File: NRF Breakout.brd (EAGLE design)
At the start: 50 x 49 mm, 58 parts, among them Q1 BSS123, Q2 BSS123, Q3 BSS123, Q4 BSS123

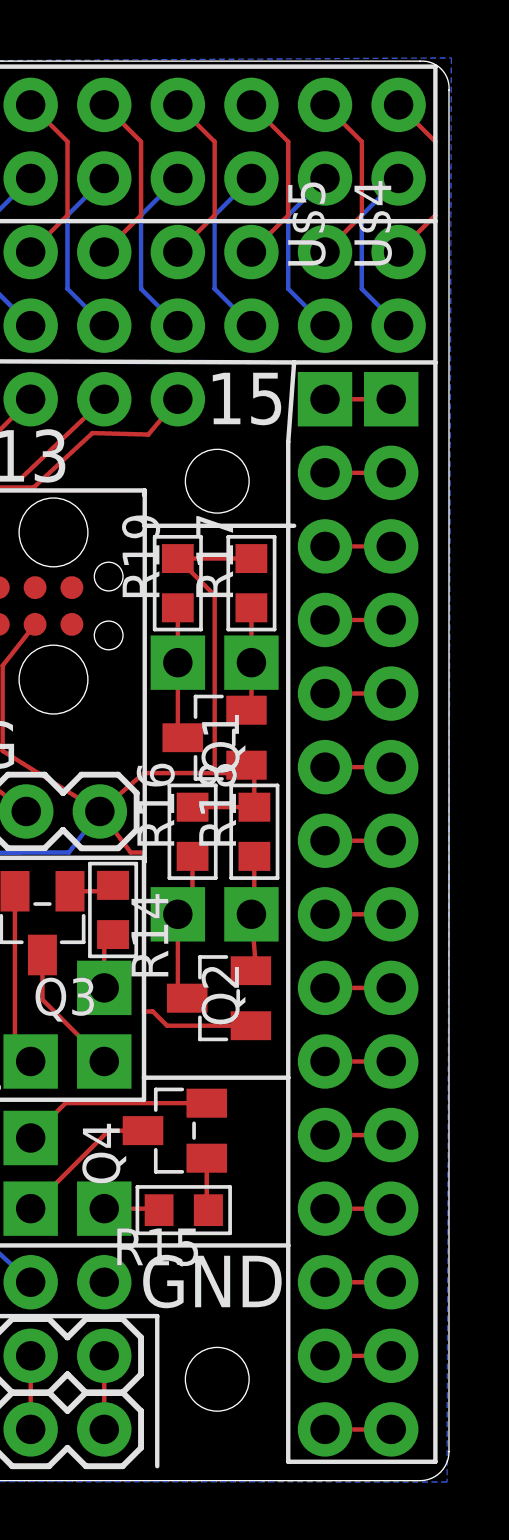
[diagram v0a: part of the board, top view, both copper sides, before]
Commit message: Continued work. This is the version that was ordered from Seeed Studios.
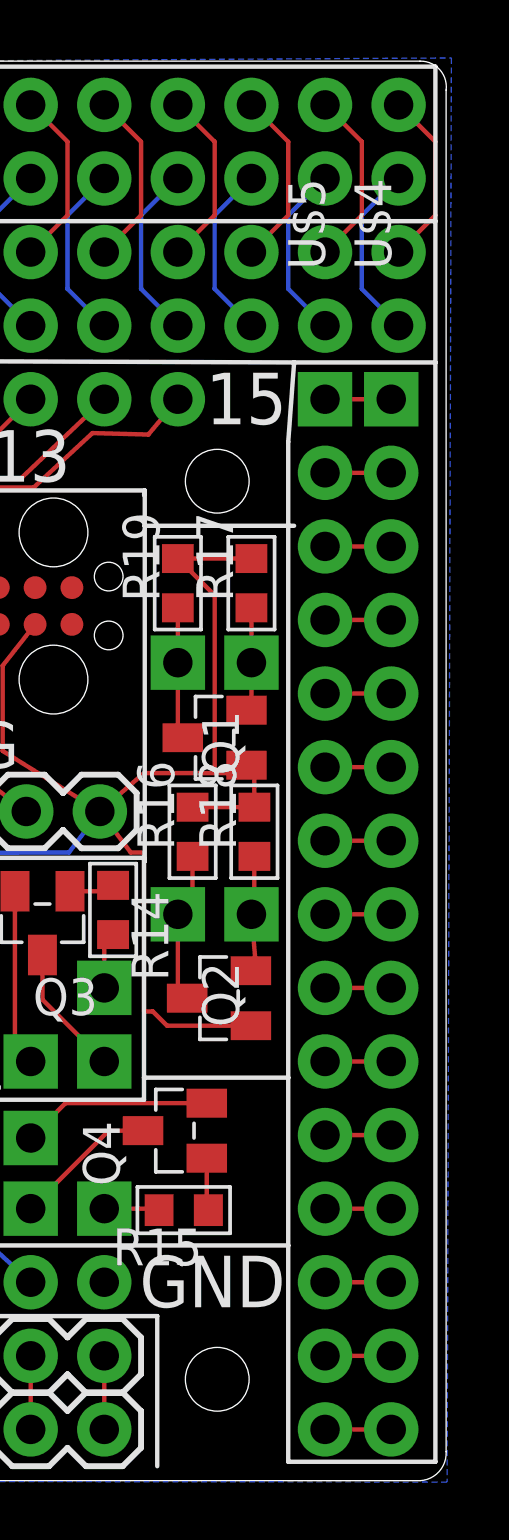
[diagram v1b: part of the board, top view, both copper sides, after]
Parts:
- Q3, Q4: value BSS123 -> MOSFET-P-TOSHIBA-SSM3J338R
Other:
- board size 50 x 49 mm -> 49.9 x 49 mm
